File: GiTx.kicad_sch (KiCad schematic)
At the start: 1 part, among them U13 XCZU15EG-2FFVB1156E

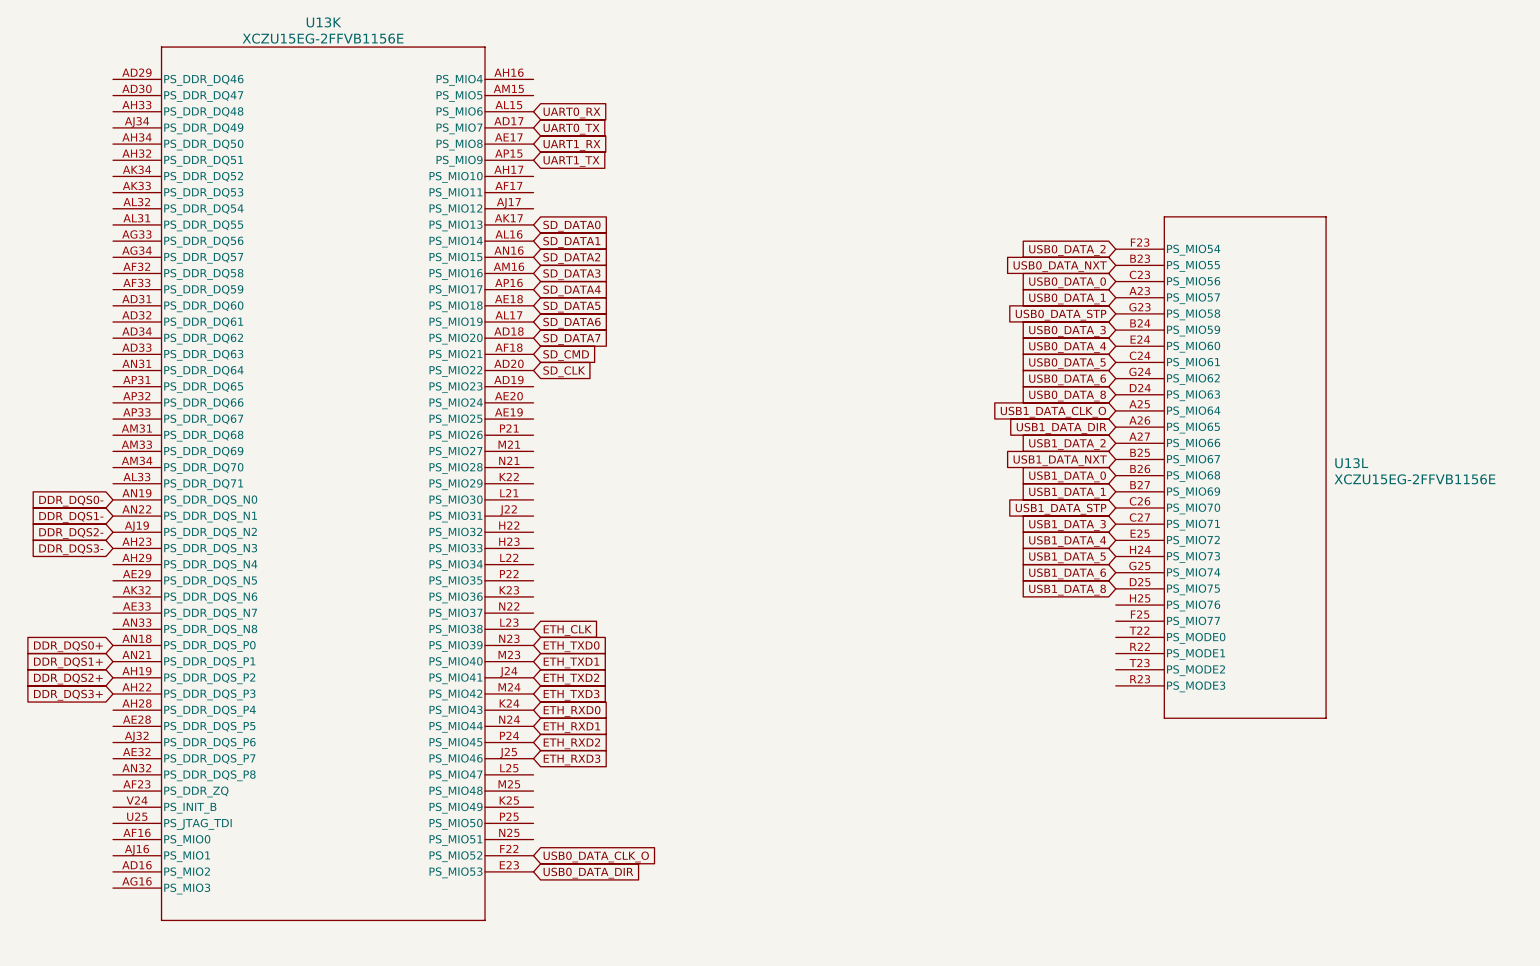
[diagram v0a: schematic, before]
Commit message: usb and stuff
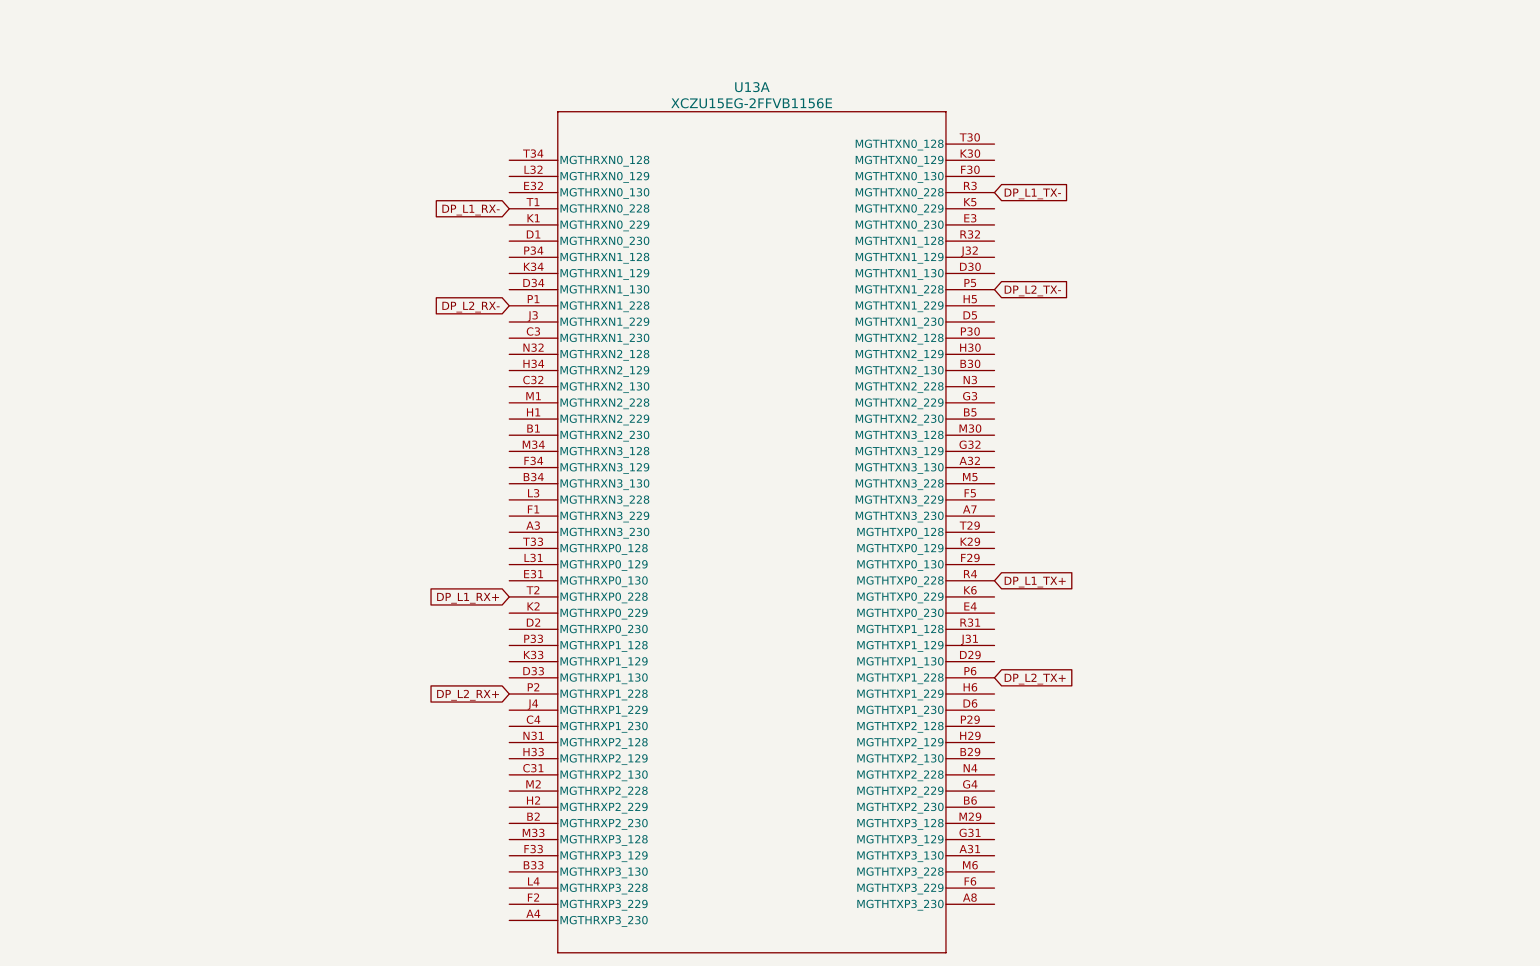
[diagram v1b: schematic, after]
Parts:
- removed U13: XCZU15EG-2FFVB1156E, lib:FFVB1156_XIL-L, symbol XCZU15EG:XCZU15EG-2FFVB1156E
- added U13: XCZU15EG-2FFVB1156E, FFVB1156_XIL, symbol XCZU15EG:XCZU15EG-2FFVB1156E
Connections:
- new net DP_L1_RX+: U13.T2 (MGTHRXP0_228)
- new net DP_L1_RX-: U13.T1 (MGTHRXN0_228)
- new net DP_L1_TX+: U13.R4 (MGTHTXP0_228)
- new net DP_L1_TX-: U13.R3 (MGTHTXN0_228)
- new net DP_L2_RX+: U13.P2 (MGTHRXP1_228)
- new net DP_L2_RX-: U13.P1 (MGTHRXN1_228)
- new net DP_L2_TX+: U13.P6 (MGTHTXP1_228)
- new net DP_L2_TX-: U13.P5 (MGTHTXN1_228)
